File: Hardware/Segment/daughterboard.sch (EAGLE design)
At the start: 163 parts, among them IC1 PBQ79656PAPTQ1, IC2 PBQ79656PAPTQ1, T1 PBHV8115X, 115, T2 PBHV8115X, 115

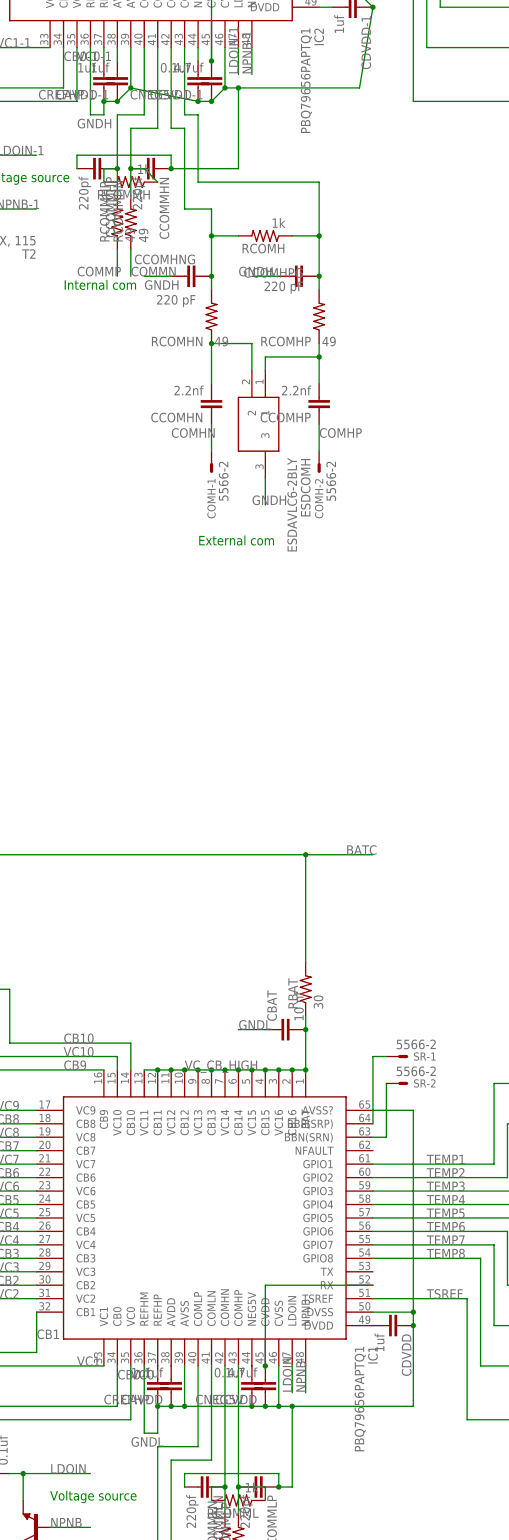
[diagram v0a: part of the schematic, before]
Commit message: Dummy battery and daughterboard v1.1
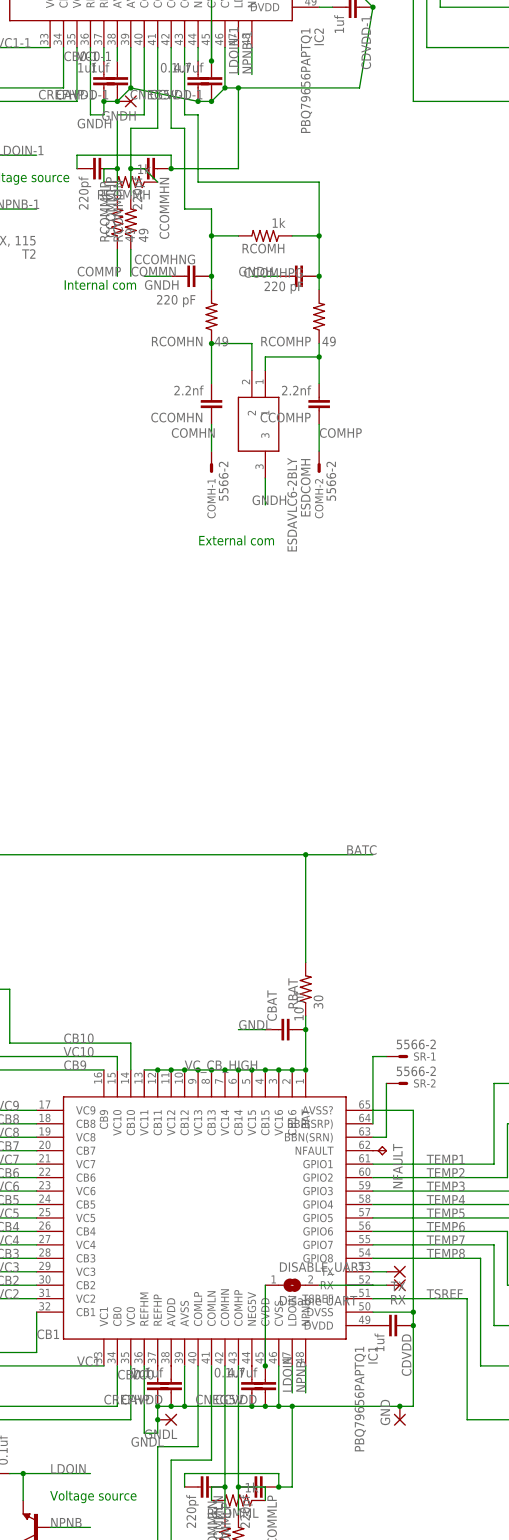
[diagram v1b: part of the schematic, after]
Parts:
- added DISABLE_UART: Disable UART, jumper:SJ
- added GND, RX, TX: (no value), wirepad:2,54/1,0
- added GNDH, GNDL: (no value), wirepad:SMD5
- added NFAULT: TPB2,54, testpad:TPB2,54
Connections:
- new net N$10: IC1.NFAULT, NFAULT.TP
- new net N$3: DISABLE_UART.2, IC1.RX, RX.P
- new net N$9: IC1.TX, TX.P
- net CVDD: now also DISABLE_UART.1; no longer IC1.RX
- net GNDH: now also GNDH.P
- net GNDL: now also GND.P, GNDL.P
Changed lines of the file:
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@@
 <part name="COMH" library="con-molex" library_urn="urn:adsk.eagle:library:165" deviceset="5566-2" device="" package3d_urn="urn:adsk.eagle:package:8078583/1"/>
 <part name="SR" library="con-molex" library_urn="urn:adsk.eagle:library:165" deviceset="5566-2" device="" package3d_urn="urn:adsk.eagle:package:8078583/1"/>
+<part name="DISABLE_UART" library="jumper" library_urn="urn:adsk.eagle:library:252" deviceset="SJ" device="" package3d_urn="urn:adsk.eagle:package:15471/1" value="Disable UART"/>
+<part name="GNDL" library="wirepad" library_urn="urn:adsk.eagle:library:412" deviceset="SMD5" device="" package3d_urn="urn:adsk.eagle:package:30841/1"/>
+<part name="GNDH" library="wirepad" library_urn="urn:adsk.eagle:library:412" deviceset="SMD5" device="" package3d_urn="urn:adsk.eagle:package:30841/1"/>
+<part name="TX" library="wirepad" library_urn="urn:adsk.eagle:library:412" deviceset="2,54/1,0" device="" package3d_urn="urn:adsk.eagle:package:30828/1"/>
+<part name="RX" library="wirepad" library_urn="urn:adsk.eagle:library:412" deviceset="2,54/1,0" device="" package3d_urn="urn:adsk.eagle:package:30828/1"/>
+<part name="GND" library="wirepad" library_urn="urn:adsk.eagle:library:412" deviceset="2,54/1,0" device="" package3d_urn="urn:adsk.eagle:package:30828/1"/>
+<part name="NFAULT" library="testpad" library_urn="urn:adsk.eagle:library:385" deviceset="TP" device="B2,54" package3d_urn="urn:adsk.eagle:package:27948/1"/>
 </parts>
 <sheets>
@@
 <attribute name="VALUE" x="194.818" y="82.677" size="1.778" layer="96"/>
 </instance>
+<instance part="DISABLE_UART" gate="1" x="175.26" y="43.18" smashed="yes">
+<attribute name="NAME" x="172.72" y="45.72" size="1.778" layer="95"/>
+<attribute name="VALUE" x="172.72" y="39.37" size="1.778" layer="96"/>
+</instance>
+<instance part="GNDL" gate="1" x="152.4" y="17.78" smashed="yes" rot="R180">
+<attribute name="NAME" x="153.543" y="15.9258" size="1.778" layer="95" rot="R180"/>
+<attribute name="VALUE" x="153.543" y="21.082" size="1.778" layer="96" rot="R180"/>
+</instance>
+<instance part="GNDH" gate="1" x="144.78" y="266.7" smashed="yes" rot="R180">
+<attribute name="NAME" x="145.923" y="264.8458" size="1.778" layer="95" rot="R180"/>
+<attribute name="VALUE" x="145.923" y="270.002" size="1.778" layer="96" rot="R180"/>
+</instance>
+<instance part="TX" gate="P" x="195.58" y="45.72" smashed="yes" rot="R180">
+<attribute name="NAME" x="196.723" y="43.8658" size="1.778" layer="95" rot="R180"/>
+<attribute name="VALUE" x="196.723" y="49.022" size="1.778" layer="96" rot="R180"/>
+</instance>
+<instance part="RX" gate="P" x="195.58" y="43.18" smashed="yes" rot="R180">
+<attribute name="NAME" x="196.723" y="41.3258" size="1.778" layer="95" rot="R180"/>
+<attribute name="VALUE" x="196.723" y="46.482" size="1.778" layer="96" rot="R180"/>
+</instance>
+<instance part="GND" gate="P" x="195.58" y="17.78" smashed="yes" rot="R90">
+<attribute name="NAME" x="193.7258" y="16.637" size="1.778" layer="95" rot="R90"/>
+<attribute name="VALUE" x="198.882" y="16.637" size="1.778" layer="96" rot="R90"/>
+</instance>
+<instance part="NFAULT" gate="G$1" x="193.04" y="68.58" smashed="yes" rot="R270">
+<attribute name="NAME" x="194.31" y="69.85" size="1.778" layer="95" rot="R270"/>
+<attribute name="TP_SIGNAL_NAME" x="191.77" y="67.31" size="1.778" layer="97" rot="R270"/>
+</instance>
 </instances>
 <busses>
@@
 <pinref part="CREFHP" gate="G$1" pin="1"/>
 <wire x1="147.32" y1="15.24" x2="149.86" y2="15.24" width="0.1524" layer="91"/>
-<wire x1="149.86" y1="15.24" x2="149.86" y2="20.32" width="0.1524" layer="91"/>
+<wire x1="149.86" y1="15.24" x2="149.86" y2="17.78" width="0.1524" layer="91"/>
 <pinref part="IC1" gate="G$1" pin="AVSS"/>
+<wire x1="149.86" y1="17.78" x2="149.86" y2="20.32" width="0.1524" layer="91"/>
 <wire x1="154.94" y1="27.94" x2="154.94" y2="20.32" width="0.1524" layer="91"/>
 <pinref part="CAVDD" gate="G$1" pin="1"/>
@@
 <wire x1="198.12" y1="38.1" x2="198.12" y2="35.56" width="0.1524" layer="91"/>
 <wire x1="198.12" y1="35.56" x2="198.12" y2="20.32" width="0.1524" layer="91"/>
-<wire x1="198.12" y1="20.32" x2="175.26" y2="20.32" width="0.1524" layer="91"/>
+<wire x1="198.12" y1="20.32" x2="195.58" y2="20.32" width="0.1524" layer="91"/>
 <junction x="198.12" y="35.56"/>
 <junction x="172.72" y="20.32"/>
 <pinref part="IC1" gate="G$1" pin="AVSS?"/>
+<wire x1="195.58" y1="20.32" x2="175.26" y2="20.32" width="0.1524" layer="91"/>
 <wire x1="175.26" y1="20.32" x2="172.72" y2="20.32" width="0.1524" layer="91"/>
 <wire x1="190.5" y1="76.2" x2="198.12" y2="76.2" width="0.1524" layer="91"/>
@@
 <junction x="172.72" y="5.08"/>
 <junction x="175.26" y="20.32"/>
+<pinref part="GNDL" gate="1" pin="P"/>
+<junction x="149.86" y="17.78"/>
+<pinref part="GND" gate="P" pin="P"/>
+<junction x="195.58" y="20.32"/>
 </segment>
 <segment>
@@
 <net name="CVDD" class="0">
 <segment>
-<pinref part="IC1" gate="G$1" pin="RX"/>
-<wire x1="190.5" y1="43.18" x2="170.18" y2="43.18" width="0.1524" layer="91"/>
 <pinref part="CCVDD" gate="G$1" pin="2"/>
 <pinref part="IC1" gate="G$1" pin="CVDD"/>
 <wire x1="170.18" y1="43.18" x2="170.18" y2="27.94" width="0.1524" layer="91"/>
 <junction x="170.18" y="27.94"/>
+<pinref part="DISABLE_UART" gate="1" pin="1"/>
 </segment>
 </net>
@@
 <net name="CVDD-1" class="0">
 <segment>
-<pinref part="IC2" gate="G$1" pin="RX"/>
-<wire x1="180.34" y1="292.1" x2="160.02" y2="292.1" width="0.1524" layer="91"/>
 <pinref part="CCVDD-1" gate="G$1" pin="2"/>
 <pinref part="IC2" gate="G$1" pin="CVDD"/>
@@
 <junction x="160.02" y="274.32"/>
 <wire x1="160.02" y1="274.32" x2="160.02" y2="276.86" width="0.1524" layer="91"/>
+<pinref part="IC2" gate="G$1" pin="RX"/>
+<wire x1="180.34" y1="292.1" x2="160.02" y2="292.1" width="0.1524" layer="91"/>
 </segment>
 </net>
@@
 <junction x="152.4" y="254"/>
 <junction x="165.1" y="269.24"/>
+<pinref part="GNDH" gate="1" pin="P"/>
 </segment>
 <segment>
@@
 </segment>
 </net>
+<net name="N$3" class="0">
+<segment>
+<pinref part="DISABLE_UART" gate="1" pin="2"/>
+<pinref part="IC1" gate="G$1" pin="RX"/>
+<wire x1="180.34" y1="43.18" x2="190.5" y2="43.18" width="0.1524" layer="91"/>
+<wire x1="193.04" y1="43.18" x2="190.5" y2="43.18" width="0.1524" layer="91"/>
+<pinref part="RX" gate="P" pin="P"/>
+</segment>
+</net>
+<net name="N$9" class="0">
+<segment>
+<pinref part="IC1" gate="G$1" pin="TX"/>
+<wire x1="193.04" y1="45.72" x2="190.5" y2="45.72" width="0.1524" layer="91"/>
+<pinref part="TX" gate="P" pin="P"/>
+</segment>
+</net>
+<net name="N$10" class="0">
+<segment>
+<pinref part="IC1" gate="G$1" pin="NFAULT"/>
+<pinref part="NFAULT" gate="G$1" pin="TP"/>
+</segment>
+</net>
